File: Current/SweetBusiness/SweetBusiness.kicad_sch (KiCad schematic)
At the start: 43 parts, among them J0 USB, J2 I2C, J3 Bridge, U0 STM32F411RETx, U1 LDO-3.3, Y1 8MHz

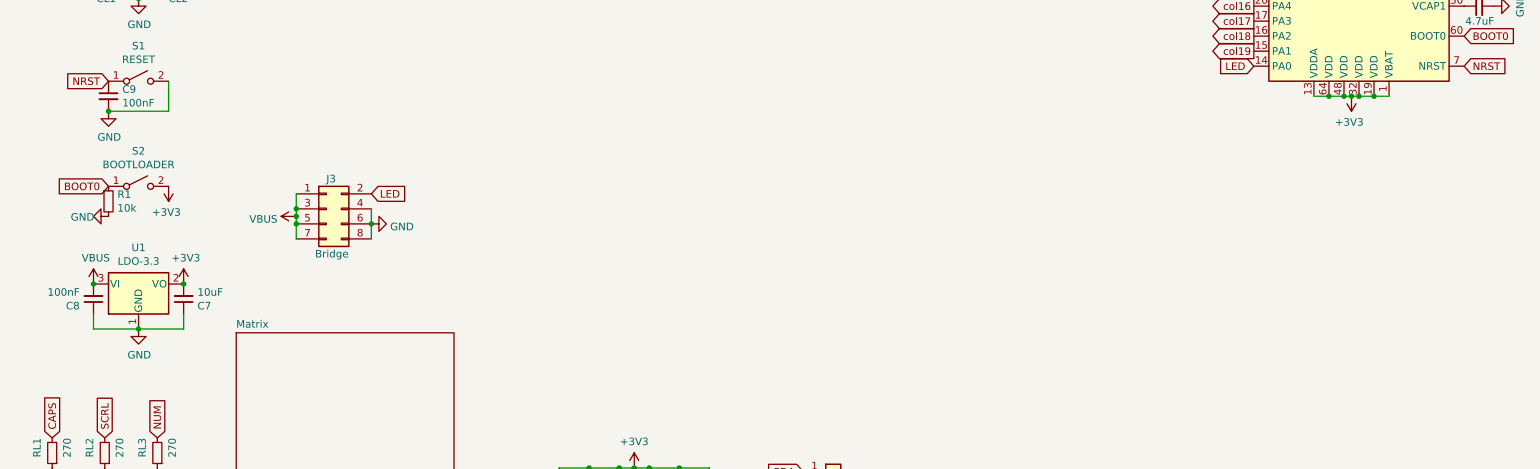
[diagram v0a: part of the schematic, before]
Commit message: oh my god just stop
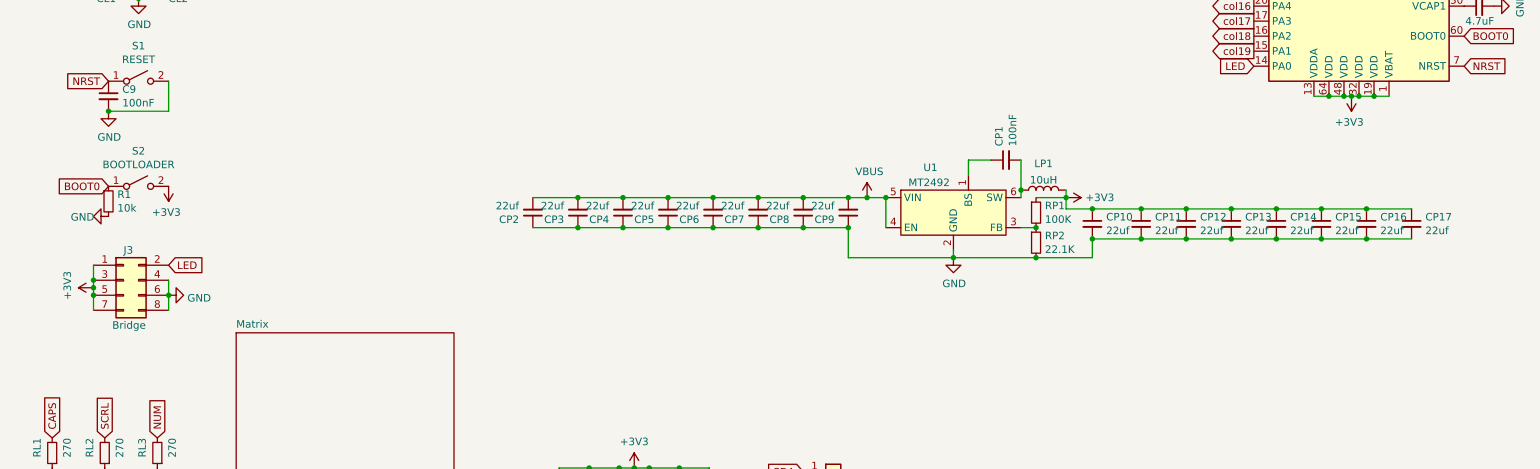
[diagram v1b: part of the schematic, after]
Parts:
- removed C7: 10uF, EDI:Passive_0402_1005Metric, symbol Device:C_Small
- removed U1: LDO-3.3, Package_TO_SOT_SMD:SOT-23, symbol Regulator_Linear:LD1117S33TR_SOT223
- added CP1: 100nF, EDI:Passive_0402_1005Metric, symbol Device:C_Small
- added CP10, CP11, CP12, CP13, CP14, CP15, CP16, CP17, CP2, CP3, CP4, CP5, CP6, CP7, CP8: 22uf, EDI:Passive_0402_1005Metric, symbol Device:C_Small
- added LP1: 10uH, Inductor_SMD:L_Wuerth_HCI-1040, symbol Device:L
- added RP1: 100K, EDI:Passive_0402_1005Metric, symbol Device:R_Small
- added RP2: 22.1K, EDI:Passive_0402_1005Metric, symbol Device:R_Small
- added U1: MT2492, Package_TO_SOT_SMD:SOT-23-6, symbol EDI:MT2492
- CP9: renamed from C8; value 100nF -> 22uf; LCSC C1525 -> C415703
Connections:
- net +3V3: now also J3.1 (Pin_1), J3.3 (Pin_3), J3.5 (Pin_5), J3.7 (Pin_7), CP10.1, CP11.1, CP12.1, CP13.1, CP14.1, CP15.1, CP16.1, CP17.1, LP1.2, RP1.1
- net GND: now also CP10.2, CP11.2, CP12.2, CP13.2, CP14.2, CP15.2, CP16.2, CP17.2, CP2.1, CP3.1, CP4.1, CP5.1, CP6.1, CP7.1, CP8.1, RP2.2, U1.2 (GND)
- net VBUS: now also CP2.2, CP3.2, CP4.2, CP5.2, CP6.2, CP7.2, CP8.2, U1.4 (EN), U1.5 (VIN); no longer J3.1 (Pin_1), J3.3 (Pin_3), J3.5 (Pin_5), J3.7 (Pin_7)
- new net: RP1.2, RP2.1, U1.3 (FB)
- new net: CP1.1, U1.1 (BS)
- new net: CP1.2, LP1.1, U1.6 (SW)
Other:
- moved on the sheet: CP9, J3
